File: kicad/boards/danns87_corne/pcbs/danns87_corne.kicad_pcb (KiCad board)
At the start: 2 copper layers, 132 x 85.7 mm, 46 parts

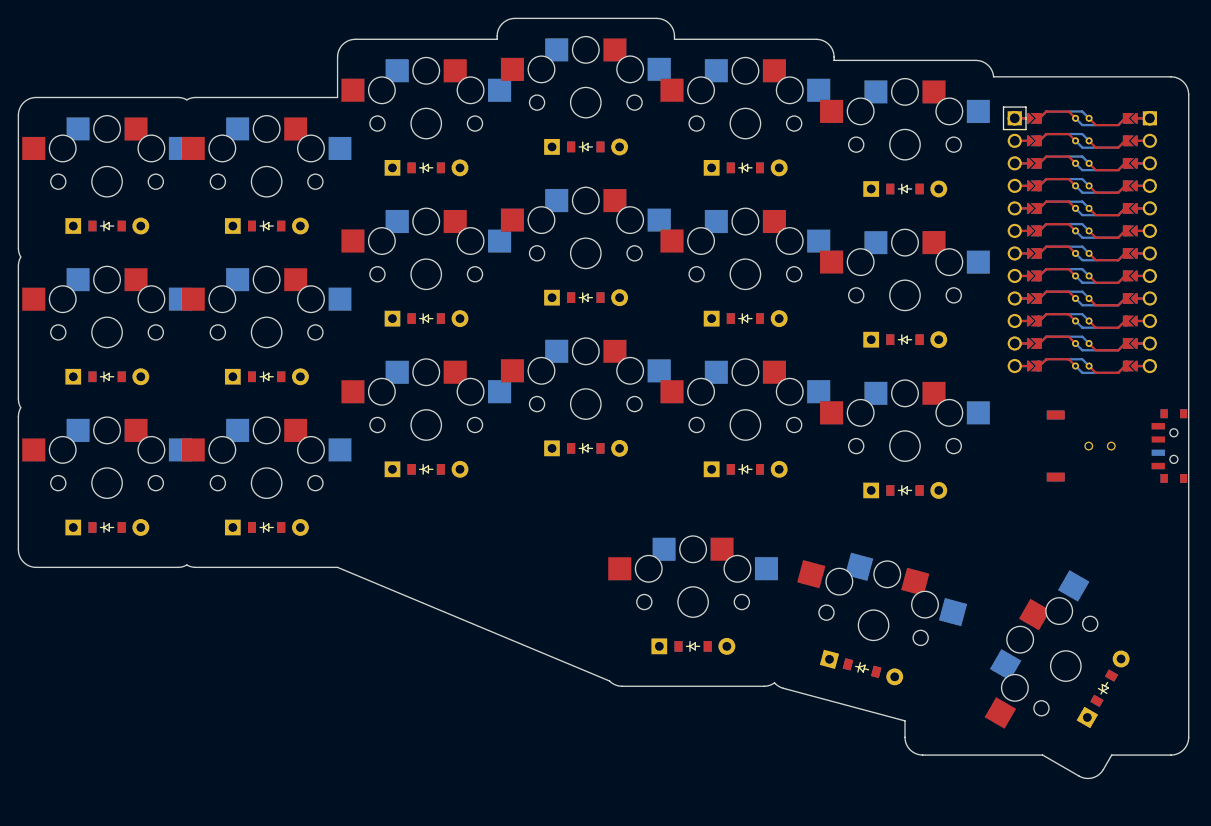
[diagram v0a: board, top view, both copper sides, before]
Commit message: danns87_corne: Almost functional
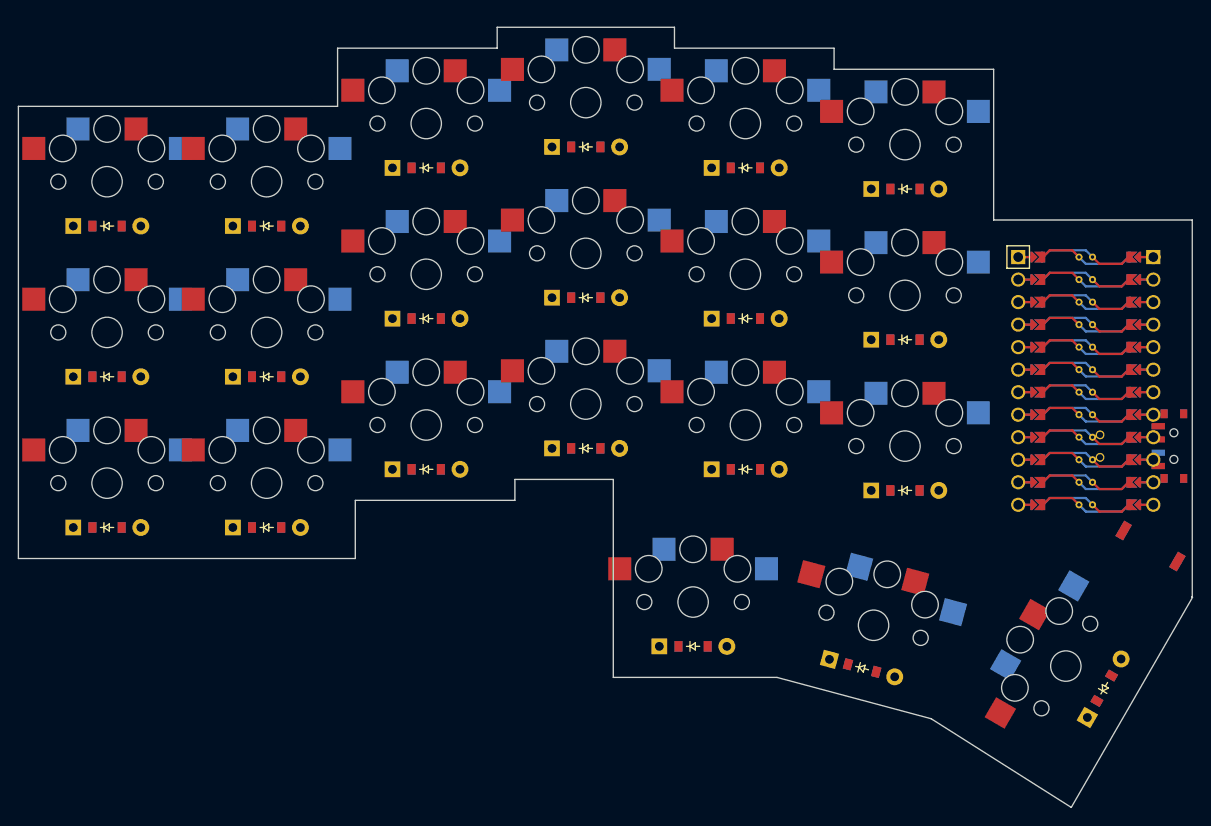
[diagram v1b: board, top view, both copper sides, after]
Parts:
- moved MCU1 15.7 mm to (128.4, -11.5)
- moved ? 15.5 mm to (135.7, 7.09), turned to 150 degrees
- turned ? to 0 degrees
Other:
- board size 132 x 85.7 mm -> 132.4 x 88 mm
